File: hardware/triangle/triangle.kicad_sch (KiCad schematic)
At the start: 59 parts, among them J1 Conn_01x02_Socket, J2 Conn_01x02_Socket

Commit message: holes only.
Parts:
- H1, H2, H3: footprint footprints:SMD_BD5.6-L5.6-W5.6-D4.1 -> MountingHole:MountingHole_3.2mm_M3; JLCPCB Part # C5301783 -> (none)
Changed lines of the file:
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@@
 			)
 		)
-		(property "Footprint" "footprints:SMD_BD5.6-L5.6-W5.6-D4.1"
+		(property "Footprint" "MountingHole:MountingHole_3.2mm_M3"
 			(at 100.965 181.61 0)
 			(hide yes)
@@
 			)
 		)
-		(property "Datasheet" "https://www.lcsc.com/product-detail/C5301783.html"
+		(property "Datasheet" ""
 			(at 100.965 181.61 0)
 			(hide yes)
@@
 			)
 		)
-		(property "JLCPCB Part #" "C5301783"
+		(property "JLCPCB Part #" ""
 			(at 100.965 181.61 0)
 			(hide yes)
@@
 			)
 		)
-		(property "Footprint" "footprints:SMD_BD5.6-L5.6-W5.6-D4.1"
+		(property "Footprint" "MountingHole:MountingHole_3.2mm_M3"
 			(at 100.965 167.64 0)
 			(hide yes)
@@
 			)
 		)
-		(property "Datasheet" "https://www.lcsc.com/product-detail/C5301783.html"
+		(property "Datasheet" ""
 			(at 100.965 167.64 0)
 			(hide yes)
@@
 			)
 		)
-		(property "JLCPCB Part #" "C5301783"
+		(property "JLCPCB Part #" ""
 			(at 100.965 167.64 0)
 			(hide yes)
@@
 			)
 		)
-		(property "Footprint" "footprints:SMD_BD5.6-L5.6-W5.6-D4.1"
+		(property "Footprint" "MountingHole:MountingHole_3.2mm_M3"
 			(at 100.965 174.625 0)
 			(hide yes)
@@
 			)
 		)
-		(property "Datasheet" "https://www.lcsc.com/product-detail/C5301783.html"
+		(property "Datasheet" ""
 			(at 100.965 174.625 0)
 			(hide yes)
@@
 			)
 		)
-		(property "JLCPCB Part #" "C5301783"
+		(property "JLCPCB Part #" ""
 			(at 100.965 174.625 0)
 			(hide yes)

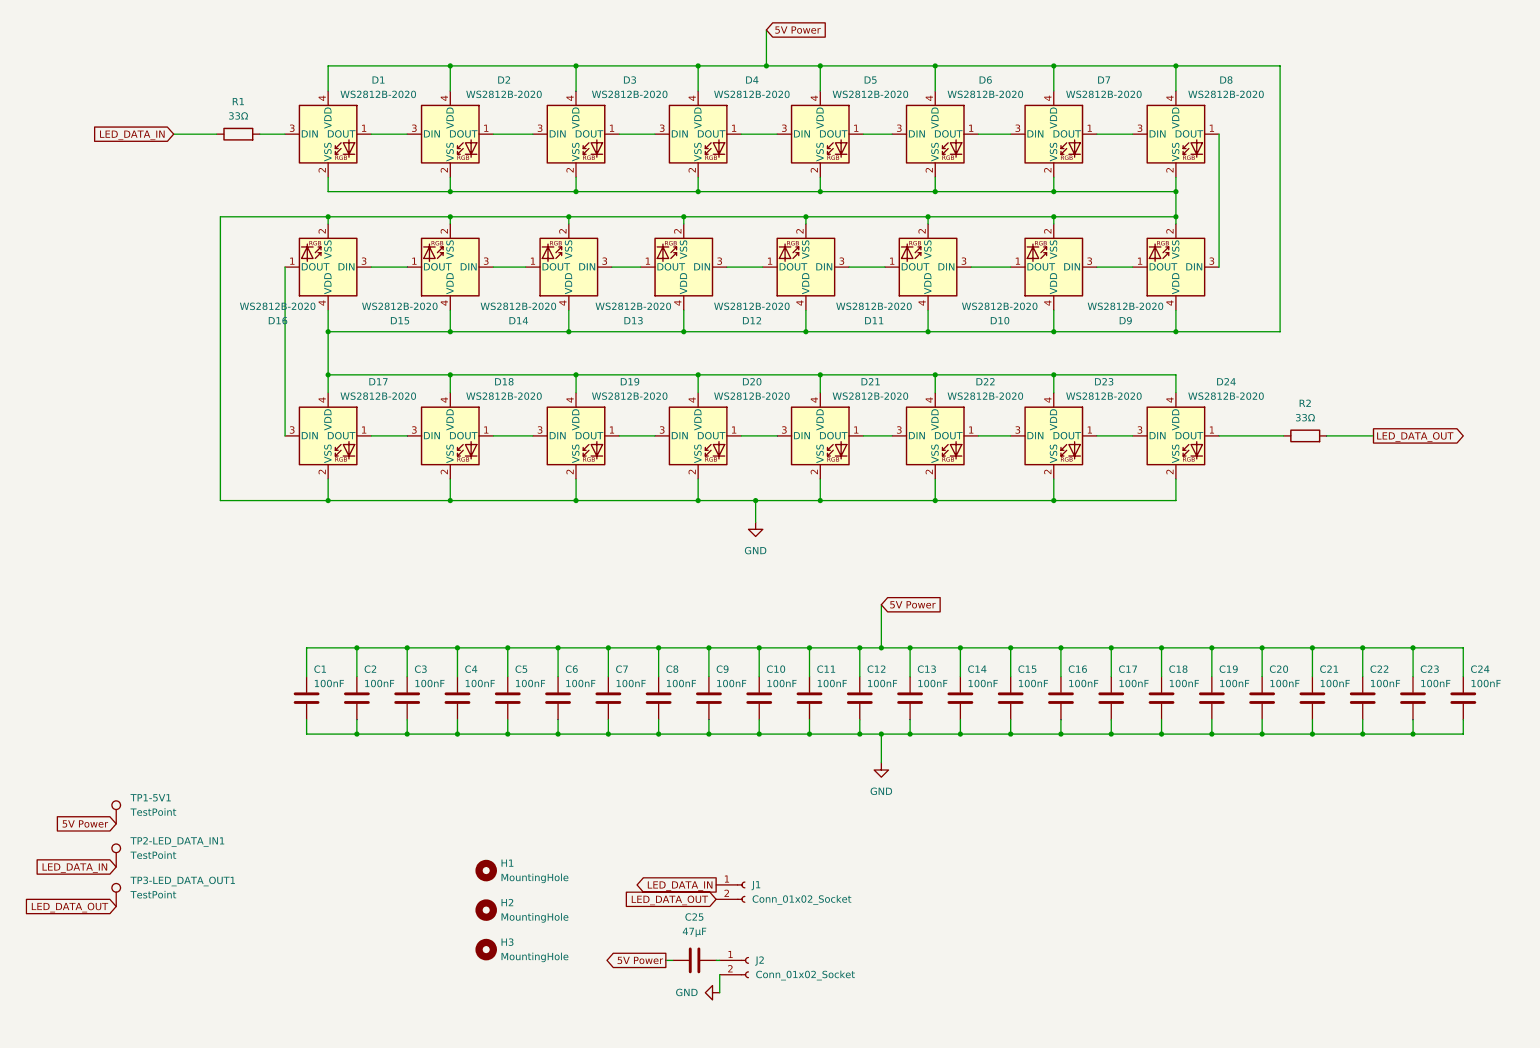
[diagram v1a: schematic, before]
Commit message: updating components on triangle board - in progress
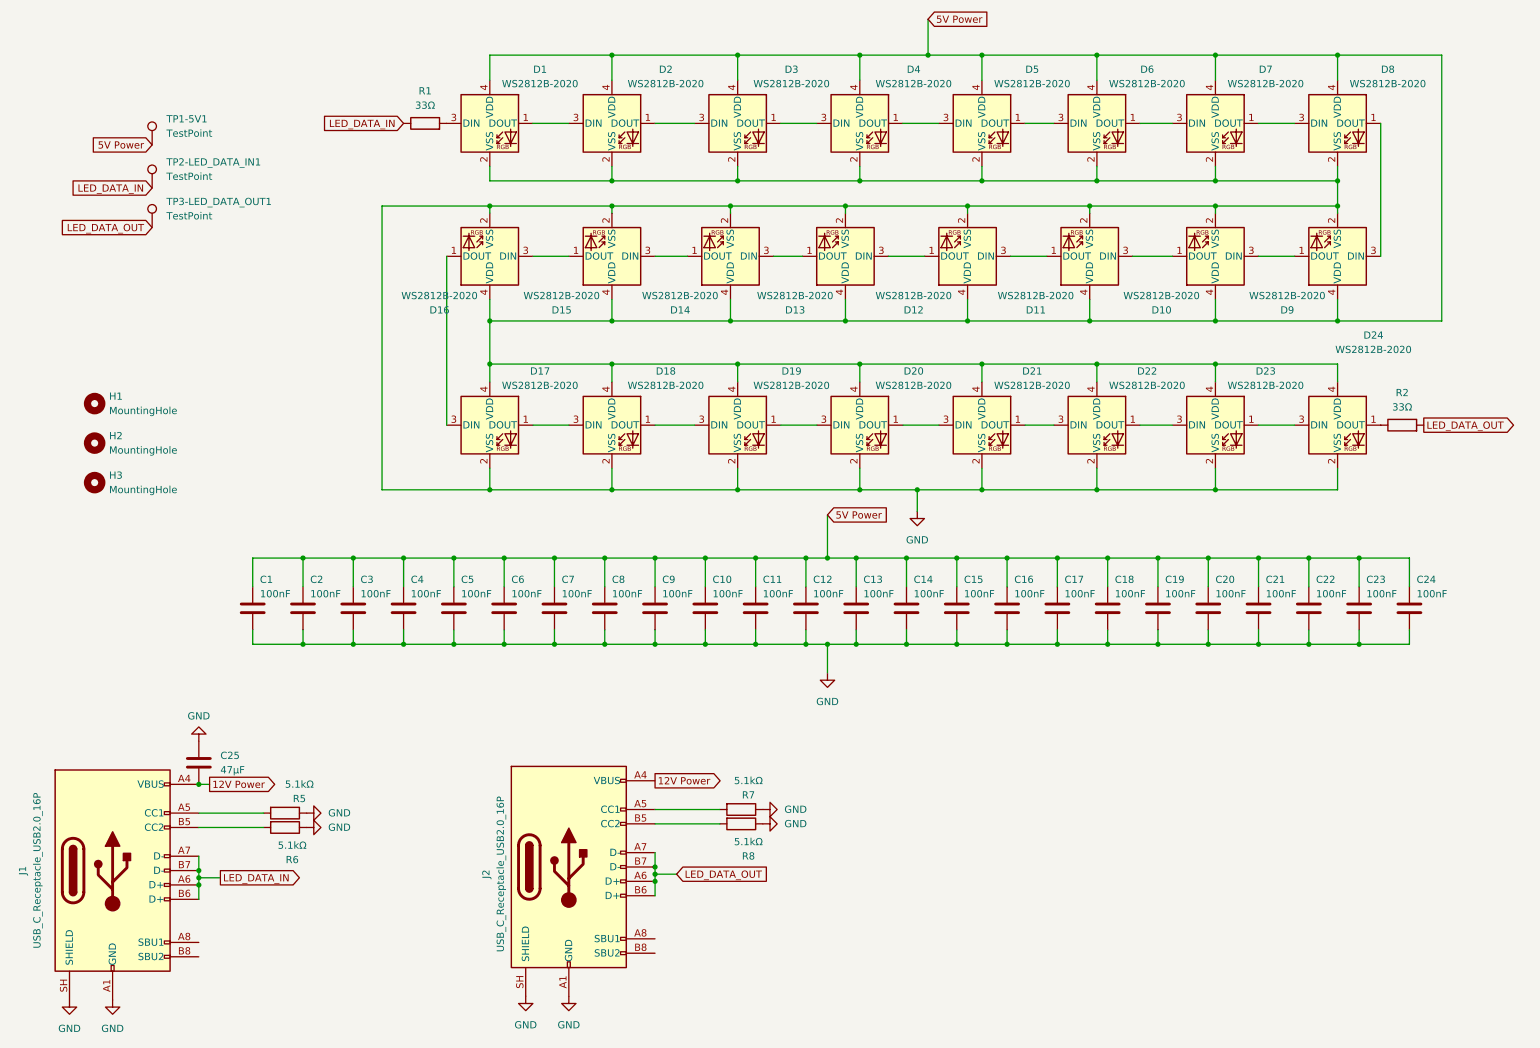
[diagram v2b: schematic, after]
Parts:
- removed J1: Conn_01x02_Socket, footprints:CONN-SMD_B2B-PH-SM4-TBT-LF-SN, symbol Connector:Conn_01x02_Socket
- removed J2: Conn_01x02_Socket, footprints:CONN-SMD_ZX-XH2.54-2PLT, symbol Connector:Conn_01x02_Socket
- added J1, J2: USB_C_Receptacle_USB2.0_16P, footprints:TYPE-C-SMD_USB4120-03-C, symbol Connector:USB_C_Receptacle_USB2.0_16P
- added R5, R6, R7, R8: 5.1kΩ, Resistor_SMD:R_0603_1608Metric, symbol Device:R
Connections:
- net 5V Power: no longer C25.1
- net GND: now also C25.1, J1.A1 (GND), J1.A12 (GND), J1.B1 (GND), J1.B12 (GND), J1.SH (SHIELD), J2.A1 (GND), J2.A12 (GND), J2.B1 (GND), J2.B12 (GND), J2.SH (SHIELD), R5.1, R6.1, R7.1, R8.1
- net LED_DATA_IN: now also J1.A6 (D+), J1.A7 (D-), J1.B6 (D+), J1.B7 (D-)
- net LED_DATA_OUT: now also J2.A6 (D+), J2.A7 (D-), J2.B6 (D+), J2.B7 (D-)
- net 12V Power: now reaches C25.2
- net 12V Power: now also J1.A4 (VBUS), J1.A9 (VBUS), J1.B4 (VBUS), J1.B9 (VBUS), J2.A4 (VBUS), J2.A9 (VBUS), J2.B4 (VBUS), J2.B9 (VBUS)
- new net: J1.B5 (CC2), R6.2
- new net: J1.A5 (CC1), R5.2
- new net: J2.A5 (CC1), R7.2
- new net: J2.B5 (CC2), R8.2
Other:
- moved on the sheet: C1, C10, C11, C12, C13, C14, C15, C16, C17, C18, C19, C2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

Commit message: trying and failing to fix the usb-c
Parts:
- TP1-5V1, TP2-LED_DATA_IN1, TP3-LED_DATA_OUT1: footprint TestPoint:TestPoint_Pad_1.0x1.0mm -> TestPoint:TestPoint_Pad_D2.0mm
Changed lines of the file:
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@@
 			)
 		)
-		(property "Footprint" "TestPoint:TestPoint_Pad_1.0x1.0mm"
+		(property "Footprint" "TestPoint:TestPoint_Pad_D2.0mm"
 			(at 46.99 39.37 0)
 			(hide yes)
@@
 			)
 		)
-		(property "Footprint" "TestPoint:TestPoint_Pad_1.0x1.0mm"
+		(property "Footprint" "TestPoint:TestPoint_Pad_D2.0mm"
 			(at 46.99 53.975 0)
 			(hide yes)
@@
 			)
 		)
-		(property "Footprint" "TestPoint:TestPoint_Pad_1.0x1.0mm"
+		(property "Footprint" "TestPoint:TestPoint_Pad_D2.0mm"
 			(at 46.99 46.99 0)
 			(hide yes)
